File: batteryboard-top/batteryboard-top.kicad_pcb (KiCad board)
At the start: 2 copper layers, 46.8 x 46.8 mm, 6 parts, among them J1 Conn_02x05_Odd_Even, J2 Conn_02x05_Odd_Even

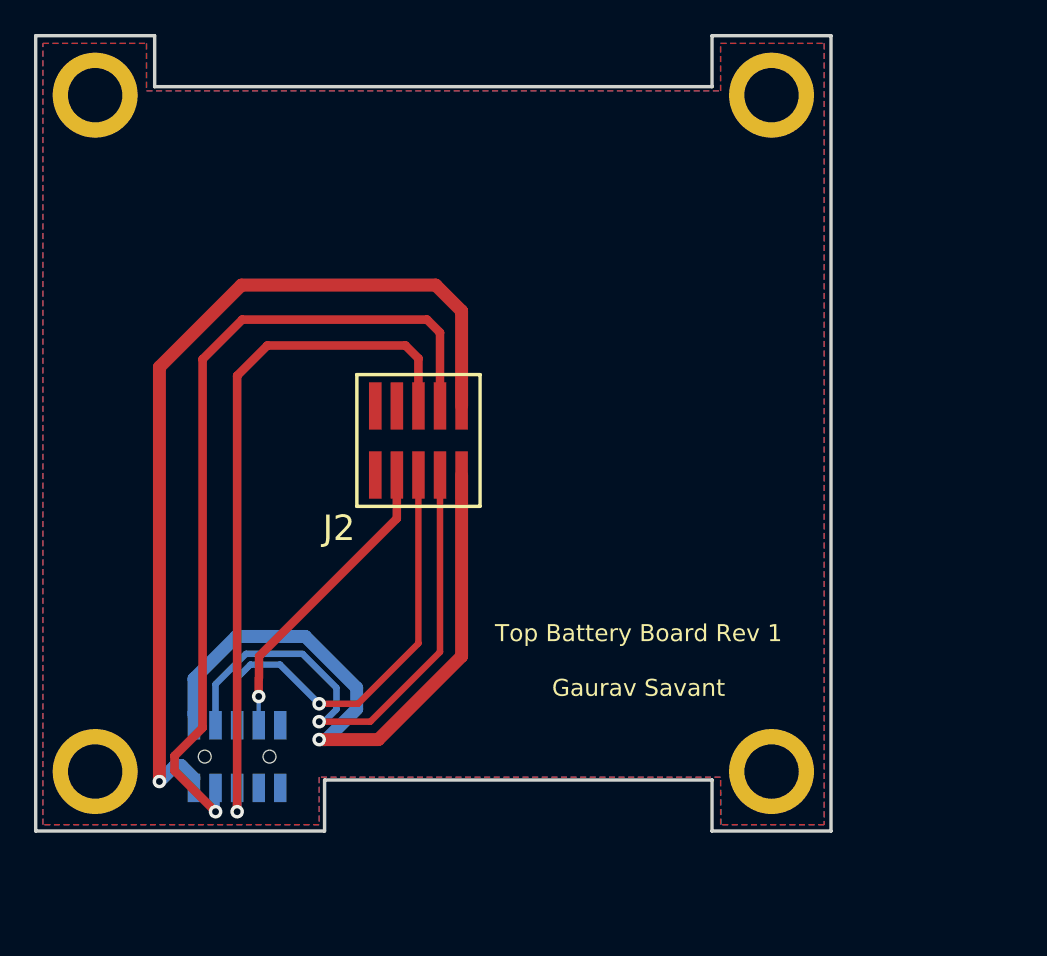
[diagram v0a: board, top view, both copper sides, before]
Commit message: Fixes and cleanup
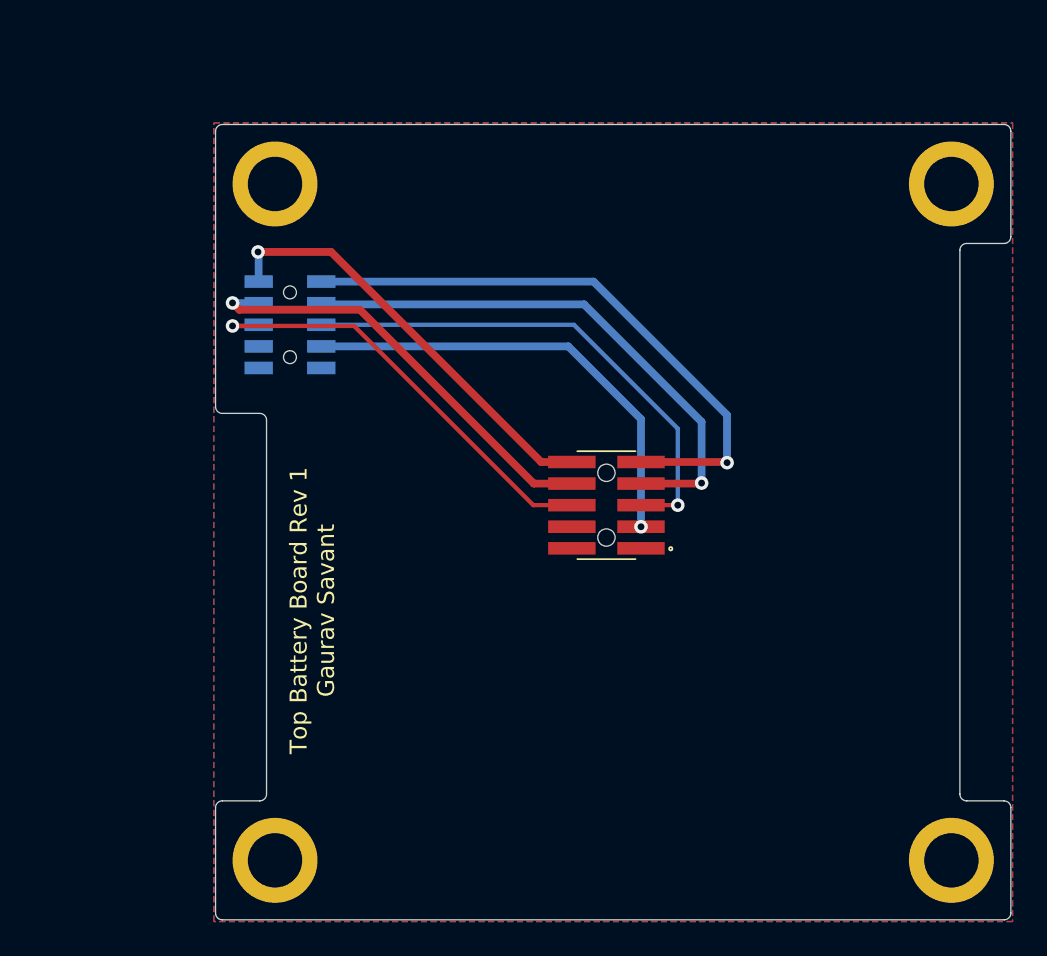
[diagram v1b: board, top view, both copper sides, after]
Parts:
- added Ref**: Val**, custom-footprints:pycubed_mini_half, F.Cu at (151.3, 75.8)
- J2: footprint batteryboard:SAMTEC-FTS-105-01-X-DV -> batteryboard:FTS-105-XX-YY-DV-A
- moved H1 50.7 mm to (170.3, 76.6), turned to -90 degrees
- moved H2 46.3 mm to (170.3, 116.4), turned to -90 degrees
- moved H4 36.2 mm to (130.5, 76.6), turned to -90 degrees
- moved H3 29.7 mm to (130.5, 116.4), turned to -90 degrees
- moved J1 25.6 mm to (131.4, 84.9), turned to 90 degrees
- moved J2 11.7 mm to (150.0, 95.5), turned to 90 degrees
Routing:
- net VBUS: track 53.1 -> 25.4 mm
- net COIL_N: track 49.8 -> 25.9 mm
- net SCL3: track 42.1 -> 25.9 mm
- net +3V3: track 18.1 -> 26.9 mm
- net SDA3: track 25.5 -> 30.2 mm
- net BATT_P: track 39.3 -> 34.9 mm
- net COIL_P: track 32.3 -> 31.8 mm
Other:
- outline, holes or cut-outs redrawn
- board text added: "09-JUN-22"
- board text added: "v01"
